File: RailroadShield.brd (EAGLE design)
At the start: 99.6 x 78.7 mm, 68 parts, among them J1 5520250-3, J2 5520250-3, J3 5520250-3, J4 5520426-4, J5 5520426-4, J6 KK-156-5, J7 KK-156-5, J8 MSTB-02, Q1 PMBT2222, U1 LM393N, U2 MCP2515-P, U3 MCP2551-P, U4 MAX3468CPA, U5 MAX3468CPA, U6 MAX3468CPA, U7 LM317LD, U8 6N137, Y1 16Mhz

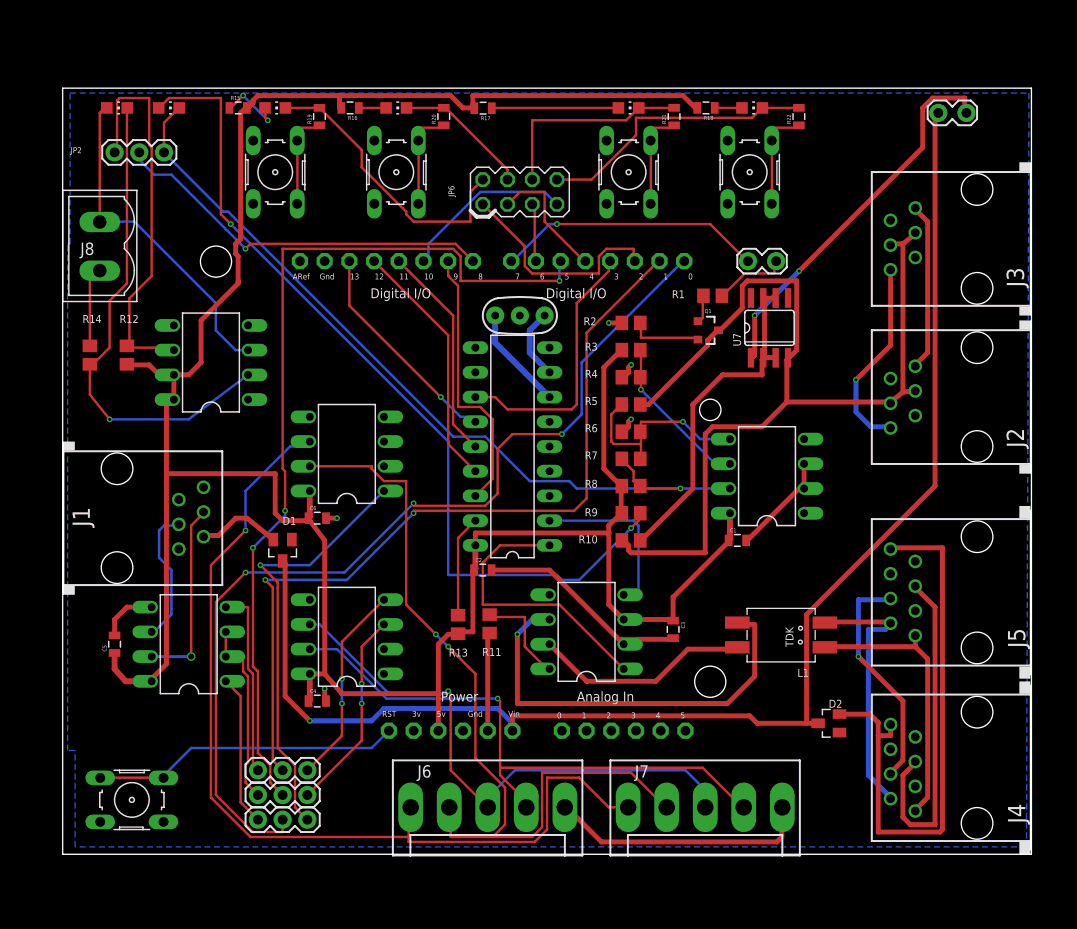
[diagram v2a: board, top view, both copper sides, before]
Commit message: 2.1smd
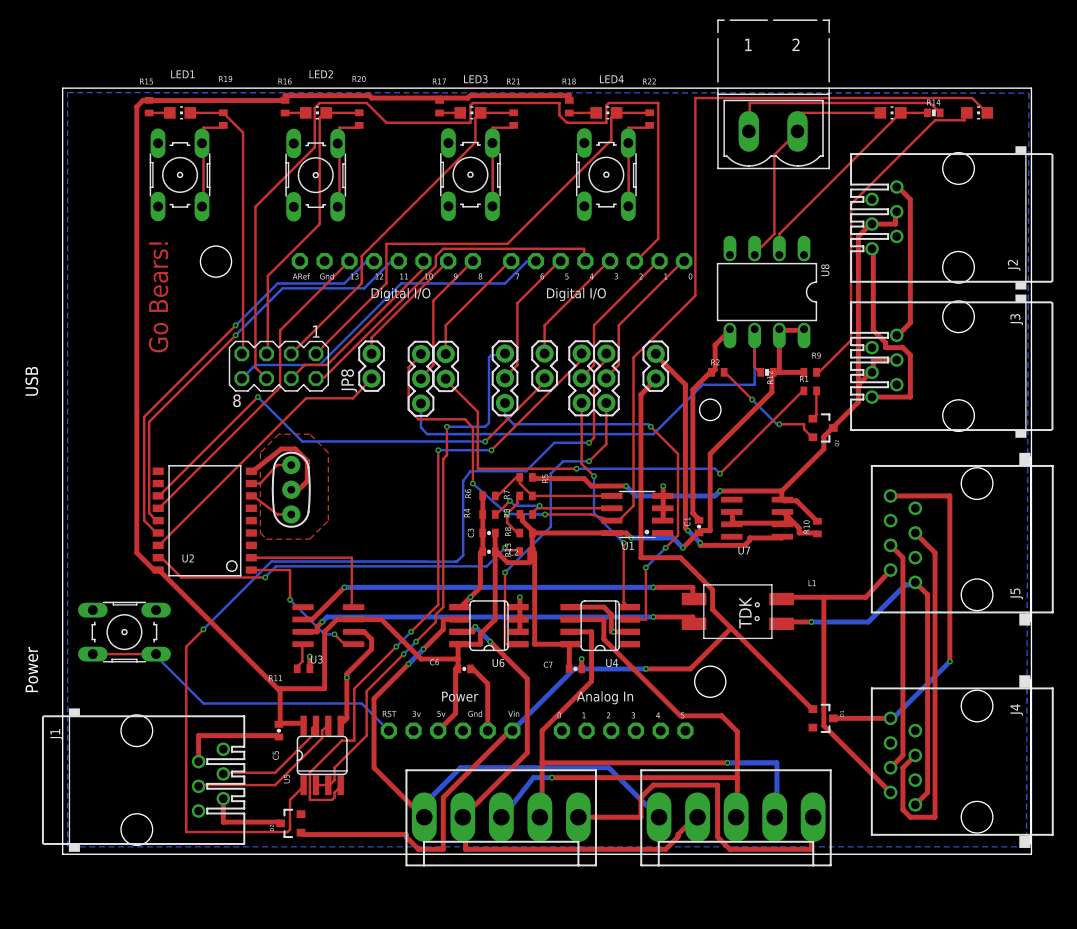
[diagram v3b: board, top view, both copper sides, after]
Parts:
- removed C4: 0.01uf, MCP:0805
- removed J8: MSTB-02, MCP:MSTBV2
- removed Q1: PMBT2222, MCP:SOT23-3
- removed U$1: ARDUINODUEMILANOVE, MCP:ARDUINO-BIGSHIELD
- added C7: .1uF, SparkFun:0402-CAP
- added J9: .200 2-pin, con-phoenix-500:MSTBV2
- added JP8: CAN-CS, SparkFun:1X02
- added JP9: (no value), con-lstb:MA04-2
- added MOD1: ARDUINO DUEMILANOVE, microbuilder:ARDUINO-BIGSHIELD
- added Q2: BC817-16LT1G, SparkFun:SOT23-3
- C1, C2, C3: value 0.01uf -> .1uf; device MCP:0805 -> SparkFun:0402-CAP
- C5, C6: value 0.01uf -> .1uF; device MCP:0805 -> SparkFun:0402-CAP
- D1, D2: value BAV199 -> (none); device diode:SOT23 -> SparkFun:SOT23-3
- J1, J2, J3: value 5520250-3 -> RJ12; device MCP:RJ11-NO_SHIELD -> con-amp:520250-3
- J4, J5: value 5520426-4 -> RJ45; device MCP:RJ45-NO-SHIELD -> con-tycoelectronics:RJ45-NO-SHIELD
- J6: value KK-156-5 -> 5-pin molex; device MCP:KK-156-5 -> con-molex:KK-156-5
- J7: value KK-156-5 -> 5-pin Molex; device MCP:KK-156-5 -> con-molex:KK-156-5
- JP1: value LN-TERM -> LN_TERM; device MCP:1X02_LOCK -> SparkFun:1X02
- JP2: device MCP:1X03 -> SparkFun:1X03
- JP3: value RxD -> CAN-INT; device MCP:1X03 -> SparkFun:1X02
- JP4: value EN -> TXD; device MCP:1X03 -> SparkFun:1X02
- JP5: value TxD -> RXD; device MCP:1X03 -> SparkFun:1X03
- JP6: value MA04-2 -> EN; device MCP:MA04-2 -> SparkFun:1X03
- JP7: value LNTX -> TXD; device MCP:1X02_LOCK -> SparkFun:1X03
- LED3, LED4: value Green -> Red
- R1, R10, R11, R13, R3, R4, R5, R6, R7, R8: device rcl:R0805 -> rcl:R0402
- R12: device rcl:R0805 -> SparkFun:0402-RES
- R14: value 1k -> 1K; device rcl:R0805 -> SparkFun:0402-RES
- R15, R16, R17, R18, R19, R20, R21, R22: value 660R -> 680R; device MCP:0805 -> rcl:R0402
- R2: value 18R -> 15R; device rcl:R0805 -> rcl:R0402
- R9: value 1k -> 1K; device rcl:R0805 -> rcl:R0402
- S1, S2, S3, S4: value B3F-1052 -> 611-PTS645SH70LFS; device MCP:B3F-10XX -> switch-omron:B3F-10XX
- S5: value B3F-1000 -> (none); device MCP:B3F-10XX -> switch-omron:B3F-10XX
- U1: value LM393N -> LM393M; device MCP:DIL08 -> MCP:SO08
- U2: value MCP2515-P -> MCP2515-SO; device MCP:DIL18 -> MCP:SO-18W
- U3: value MCP2551-P -> MCP2551-SN; device MCP:DIL08 -> MCP:SO-08
- U4, U5, U6: value MAX3468CPA -> MAX3468CSA; device MCP:DIL08 -> maxim:SO08
- U7: value LM317LD -> LM317LM; device MCP:SO08 -> linear:SO08
- Y1: device MCP:RESONATOR-PTH -> SparkFun:RESONATOR-PTH
- moved R14 90.2 mm to (89.5, 76.2), turned to 180 degrees
- moved LED6 83.1 mm to (94.0, 76.2)
- moved LED5 79.5 mm to (85.1, 76.2)
- moved R12 65.8 mm to (72.4, 49.5), turned to 0 degrees
- moved D1 58.1 mm to (78.1, 14.0), turned to 270 degrees
- moved U8 57.6 mm to (72.4, 57.8), turned to 180 degrees
- moved D2 56.2 mm to (23.5, 3.17)
- moved JP3 51.5 mm to (49.5, 48.9), turned to 90 degrees
- moved JP5 48.7 mm to (55.9, 46.4), turned to 90 degrees
- moved JP4 47.5 mm to (39.4, 51.4), turned to 270 degrees
- moved JP2 40.7 mm to (36.8, 46.3), turned to 90 degrees
- moved JP1 40.3 mm to (61.0, 51.4), turned to 270 degrees
- moved U2 32.5 mm to (14.6, 34.3)
- moved Y1 29.5 mm to (23.5, 37.5), turned to 90 degrees
- moved J1 27.0 mm to (7.62, 7.62)
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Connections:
- net N$10 renamed +IN
- net N$12 renamed OSC1
- net N$13 renamed OSC2
- net N$2 renamed L2+
- net N$3 renamed L3+
- net N$4 renamed L4+
- net N$5 renamed L1+
- net N$6 renamed SHIELD
- net N$7 renamed -OUT
- net N$8 renamed +OUT
- net N$9 renamed -IN
- removed net N$11: J8.1, R14.1
- new net CAN-CS: JP8.1, U2.16
- new net CAN-INT: JP3.1, U2.12
- new net DCCA: J9.1, R14.1
- net 3V: now also MOD1.3V; no longer U$1.3V
- net A/RESET: now also MOD1.RESET; no longer U$1.RESET
- net CAN-PWR+: now also D1.3; no longer D2.2
- net CMRIRX: now also JP5.1; no longer JP3.1
- net CMRITX: now also JP7.1; no longer JP5.1
- net CMRITXEN: now also JP6.1; no longer JP4.1
- net D0: now also JP5.2, MOD1.D0; no longer JP3.2, U$1.D0
- net D1: now also JP7.2, MOD1.D1; no longer JP5.2, U$1.D1
- net D10: now also JP9.4, MOD1.D10; no longer JP6.7, U$1.D10
- net D11: now also MOD1.D11; no longer U$1.D11
- net D12: now also MOD1.D12; no longer U$1.D12
- net D13: now also MOD1.D13; no longer U$1.D13
- net D2: now also JP9.6, MOD1.D2; no longer JP6.1, U$1.D2
- net D3: now also JP3.2, MOD1.D3; no longer U$1.D3, U2.12
- net D4: now also JP9.2, MOD1.D4; no longer JP6.3, U$1.D4
- net D5: now also JP6.2, MOD1.D5; no longer JP4.2, U$1.D5
- net D6: now also JP9.8, MOD1.D6; no longer JP6.5, U$1.D6
- net D7: now also JP4.1, MOD1.D7; no longer JP7.2, U$1.D7
- net D8: now also MOD1.D8; no longer U$1.D8
- net D9: now also JP8.2, MOD1.D9; no longer U$1.D9, U2.16
- net DCCB: now also J9.2; no longer J8.2
- net GND: now also C7.2, MOD1.GND, MOD1.GND1, MOD1.GND2; no longer C4.2, U$1.GND, U$1.GND1, U$1.GND2
- net IO1: now also JP9.7; no longer JP6.2
- net IO2: now also JP9.5; no longer JP6.4
- net IO3: now also JP9.3; no longer JP6.6
- net IO4: now also JP9.1; no longer JP6.8
- net LN-TX: now also Q2.1; no longer Q1.1
- net LNTX: now also JP4.2; no longer JP7.1
- net LOCONET: now also Q2.3; no longer Q1.3
- net N$1: now also Q2.2; no longer Q1.2
- net NCE-PWR+: now also D2.3; no longer D1.2
- net NCERX: now also JP5.3; no longer JP3.3
- net NCETX: now also JP7.3; no longer JP5.3
- net NCETXEN: now also JP6.3; no longer JP4.3
- net V+: now also D1.1, D2.1, MOD1.VIN; no longer D1.3, D2.3, U$1.VIN
- net VCC: now also C7.1, MOD1.5V; no longer C4.1, U$1.5V
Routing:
- net NCERX: track 15.6 -> 99.5 mm, vias 0 -> 2
- net D0: track 98.3 -> 15.4 mm, vias 3 -> 0
- net D5: track 92.3 -> 14.5 mm, vias 3 -> 0
- net D1: track 84.5 -> 15.4 mm, vias 2 -> 0
- net D2: track 23.1 -> 89.9 mm
- net L6+: track 88.7 -> 35.1 mm, vias 2 -> 0
- net CAN-INT: track 0.00 -> 48.7 mm, vias 0 -> 2
- net NCETX: track 19.5 -> 65.5 mm, vias 0 -> 4
- net +IN: track 97.1 -> 56.3 mm, vias 1 -> 2
- net LNTX: track 7.79 -> 47.8 mm, vias 0 -> 2
- net V+: track 142.0 -> 102.0 mm
- net GND: track 56.9 -> 94.8 mm, vias 5 -> 7
- net NCETXEN: track 19.4 -> 56.3 mm, vias 0 -> 3
- net LNRX: track 85.9 -> 118.1 mm, vias 1 -> 3
- net -IN: track 84.9 -> 55.5 mm
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- added copper zone on layer 1, net GND
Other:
- board text added: "16Mhz"
- board text added: "2010.10"
- board text added: "Activity"
- board text added: "CAN-CS"
- board text added: "D3"
- board text added: "D9"
- board text added: "Designed in the PCR / Coast Division / NMRA"
- board text added: "RXD"
- board text added: "Railroad"
- board text added: "Rev. 2.1smd"
- board text added: "Switches"
- board text added: "Termination"
- board text added: "layout interface"
- board text added: "shield"
- board text removed: ""Go Bears!""
- board text removed: "15mA Loconet Termination"
- board text removed: "2012.03"
- board text removed: "Railroadshield"
- board text removed: "Rev. 2.1"
- board text removed: "So then it's up with the Blue and Gold, Down with the Red..."
- board text removed: "layout interface board"

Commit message: 2.2
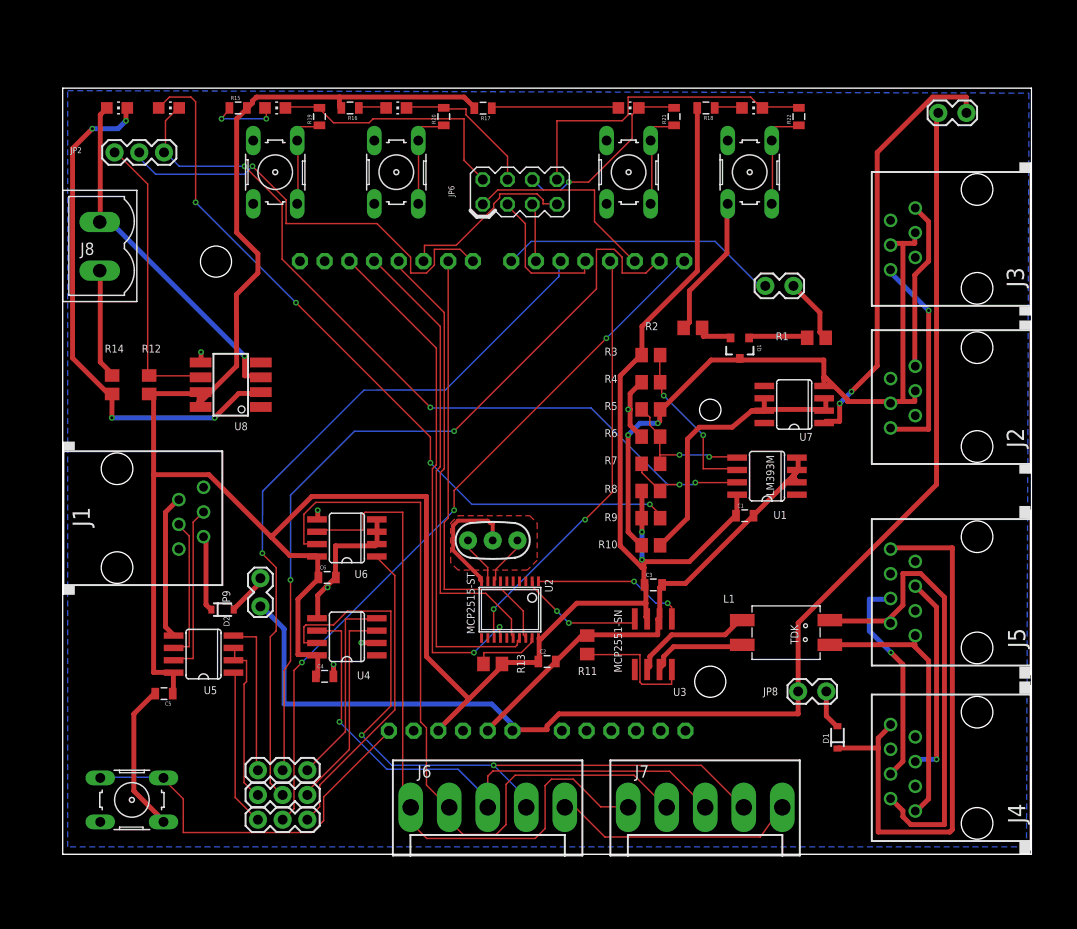
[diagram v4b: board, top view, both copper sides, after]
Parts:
- removed C7: .1uF, SparkFun:0402-CAP
- removed J9: .200 2-pin, con-phoenix-500:MSTBV2
- removed MOD1: ARDUINO DUEMILANOVE, microbuilder:ARDUINO-BIGSHIELD
- removed Q2: BC817-16LT1G, SparkFun:SOT23-3
- added C4: 0.01uf, MCP:0805
- added J8: MSTB-02, MCP:MSTBV2
- added Q1: PMBT2222, MCP:SOT23-3
- added U$1: ARDUINODUEMILANOVE, MCP:ARDUINO-BIGSHIELD
- C1, C2, C3: value .1uf -> 0.01uf; device SparkFun:0402-CAP -> MCP:0805
- C5, C6: value .1uF -> 0.01uf; device SparkFun:0402-CAP -> MCP:0805
- D1, D2: value (none) -> 1N4448WT; device SparkFun:SOT23-3 -> MCP:SOD-323
- J1, J2, J3: value RJ12 -> 5520250-3; device con-amp:520250-3 -> MCP:RJ11-NO_SHIELD
- J4, J5: value RJ45 -> 5520426-4; device con-tycoelectronics:RJ45-NO-SHIELD -> MCP:RJ45-NO-SHIELD
- J6: value 5-pin molex -> KK-156-5; device con-molex:KK-156-5 -> MCP:KK-156-5
- J7: value 5-pin Molex -> KK-156-5; device con-molex:KK-156-5 -> MCP:KK-156-5
- JP1: value LN_TERM -> LN-TERM; device SparkFun:1X02 -> MCP:1X02_LOCK
- JP2: device SparkFun:1X03 -> MCP:1X03
- JP3: value CAN-INT -> RxD; device SparkFun:1X02 -> MCP:1X03
- JP4: value TXD -> EN; device SparkFun:1X02 -> MCP:1X03
- JP5: value RXD -> TxD; device SparkFun:1X03 -> MCP:1X03
- JP6: value EN -> MA04-2; device SparkFun:1X03 -> MCP:MA04-2
- JP7: value TXD -> LNTX; device SparkFun:1X03 -> MCP:1X02_LOCK
- JP8: value CAN-CS -> CANPWR; device SparkFun:1X02 -> MCP:1X02_LOCK
- JP9: value (none) -> NCEPWR; device con-lstb:MA04-2 -> MCP:1X02_LOCK
- LED3, LED4: value Red -> Green
- R1, R10, R11, R13, R3, R4, R5, R6, R7, R8: device rcl:R0402 -> rcl:R0805
- R12: device SparkFun:0402-RES -> rcl:R0805
- R14: value 1K -> 1k; device SparkFun:0402-RES -> rcl:R0805
- R15, R16, R17, R18, R19, R20, R21, R22: value 680R -> 660R; device rcl:R0402 -> MCP:0805
- R2: value 15R -> 18R; device rcl:R0402 -> rcl:R0805
- R9: value 1K -> 1k; device rcl:R0402 -> rcl:R0805
- S1, S2, S3, S4: value 611-PTS645SH70LFS -> B3F-1052; device switch-omron:B3F-10XX -> MCP:B3F-10XX
- S5: value (none) -> B3F-1000; device switch-omron:B3F-10XX -> MCP:B3F-10XX
- U2: value MCP2515-SO -> MCP2515-ST; device MCP:SO-18W -> MCP:TSSOP20
- U4, U5, U6: device maxim:SO08 -> MCP:SO08
- U7: value LM317LM -> LM317LCDR; device linear:SO08 -> MCP:SO08
- U8: value 6N137 -> 6N137SD; device optocoupler:DIL08 -> MCP:SM8
- Y1: device SparkFun:RESONATOR-PTH -> MCP:RESONATOR-PTH
- moved R14 89.0 mm to (5.08, 48.3), turned to 270 degrees
- moved LED6 83.1 mm to (10.9, 76.7)
- moved LED5 79.5 mm to (5.59, 76.7)
- moved R12 63.5 mm to (8.89, 48.3), turned to 270 degrees
- moved JP8 56.6 mm to (78.3, 16.7), turned to 180 degrees
- moved U8 55.9 mm to (17.3, 48.3), turned to 90 degrees
- moved JP3 51.5 mm to (25.1, 3.56), turned to 180 degrees
- moved JP5 48.7 mm to (25.1, 8.64), turned to 180 degrees
- moved JP4 47.5 mm to (25.1, 6.10), turned to 180 degrees
- moved JP2 40.7 mm to (5.33, 72.1), turned to 0 degrees
- moved JP1 40.3 mm to (92.7, 76.2), turned to 180 degrees
- moved U3 33.5 mm to (60.7, 21.6), turned to 180 degrees
- moved U2 32.7 mm to (46.0, 25.1), turned to 180 degrees
- moved R11 29.3 mm to (53.9, 21.5), turned to 90 degrees
- moved J1 27.0 mm to (5.59, 34.5)
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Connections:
- net +IN renamed N$10
- net +OUT renamed N$8
- net -IN renamed N$9
- net -OUT renamed N$7
- net L1+ renamed N$5
- net L2+ renamed N$2
- net L3+ renamed N$3
- net L4+ renamed N$4
- net SHIELD renamed N$6
- removed net CAN-CS: JP8.1, U2.16
- removed net CAN-INT: JP3.1, U2.12
- removed net DCCA: J9.1, R14.1
- removed net OSC1: U2.8, Y1.3
- removed net OSC2: U2.7, Y1.1
- new net N$11: J8.1, R14.1
- new net N$12: U2.9, Y1.3
- new net N$13: U2.8, Y1.1
- new net N$14: D2.2, JP9.1
- new net N$15: D1.2, JP8.1
- net /RESET: now also U2.19; no longer U2.17
- net 3V: now also U$1.3V; no longer MOD1.3V
- net A/RESET: now also U$1.RESET; no longer MOD1.RESET
- net CAN-PWR+: now also D1.1; no longer D1.3
- net CMRIRX: now also JP3.1; no longer JP5.1
- net CMRITX: now also JP5.1; no longer JP7.1
- net CMRITXEN: now also JP4.1; no longer JP6.1
- net D0: now also JP3.2, U$1.D0; no longer JP5.2, MOD1.D0
- net D1: now also JP5.2, U$1.D1; no longer JP7.2, MOD1.D1
- net D10: now also JP6.7, U$1.D10; no longer JP9.4, MOD1.D10
- net D11: now also U$1.D11, U2.16; no longer MOD1.D11, U2.14
- net D12: now also U$1.D12, U2.17; no longer MOD1.D12, U2.15
- net D13: now also U$1.D13, U2.14; no longer MOD1.D13, U2.13
- net D2: now also JP6.1, U$1.D2; no longer JP9.6, MOD1.D2
- net D3: now also U$1.D3, U2.13; no longer JP3.2, MOD1.D3
- net D4: now also JP6.3, U$1.D4; no longer JP9.2, MOD1.D4
- net D5: now also JP4.2, U$1.D5; no longer JP6.2, MOD1.D5
- net D6: now also JP6.5, U$1.D6; no longer JP9.8, MOD1.D6
- net D7: now also JP7.2, U$1.D7; no longer JP4.1, MOD1.D7
- net D8: now also U$1.D8; no longer MOD1.D8
- net D9: now also U$1.D9, U2.18; no longer JP8.2, MOD1.D9
- net DCCB: now also J8.2; no longer J9.2
- net GND: now also C4.2, U$1.GND, U$1.GND1, U$1.GND2, U2.10; no longer C7.2, MOD1.GND, MOD1.GND1, MOD1.GND2, U2.9
- net IO1: now also JP6.2; no longer JP9.7
- net IO2: now also JP6.4; no longer JP9.5
- net IO3: now also JP6.6; no longer JP9.3
- net IO4: now also JP6.8; no longer JP9.1
- net LN-TX: now also Q1.1; no longer Q2.1
- net LNTX: now also JP7.1; no longer JP4.2
- net LOCONET: now also Q1.3; no longer Q2.3
- net N$1: now also Q1.2; no longer Q2.2
- net NCE-PWR+: now also D2.1; no longer D2.3
- net NCERX: now also JP3.3; no longer JP5.3
- net NCETX: now also JP5.3; no longer JP7.3
- net NCETXEN: now also JP4.3; no longer JP6.3
- net V+: now also JP8.2, JP9.2, U$1.VIN; no longer D1.1, D2.1, MOD1.VIN
- net VCC: now also C4.1, U$1.5V, U2.20; no longer C7.1, MOD1.5V, U2.18
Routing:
- net NCERX: track 99.5 -> 16.2 mm, vias 2 -> 0
- net D2: track 89.9 -> 21.2 mm
- net D1: track 15.4 -> 81.8 mm, vias 0 -> 2
- net D5: track 14.5 -> 73.9 mm, vias 0 -> 1
- net D0: track 15.4 -> 74.6 mm, vias 0 -> 3
- net NCETX: track 65.5 -> 16.2 mm, vias 4 -> 0
- net CAN-INT: track 48.7 -> 0.00 mm, vias 2 -> 0
- net L6+: track 35.1 -> 77.8 mm, vias 0 -> 4
- net LNTX: track 47.8 -> 6.71 mm, vias 2 -> 0
- net NCETXEN: track 56.3 -> 17.3 mm, vias 3 -> 0
- net VCC: track 244.3 -> 283.1 mm
- net GND: track 94.8 -> 133.1 mm, vias 7 -> 6
- net D9: track 12.8 -> 45.8 mm
- net /RESET: track 39.6 -> 7.00 mm, vias 2 -> 0
- net V+: track 102.0 -> 134.2 mm, vias 1 -> 0
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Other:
- board text added: ""Go Bears!""
- board text added: "Loconet Termination Power"
- board text added: "Railroadshield"
- board text added: "Rev. 2.2"
- board text added: "So then it's up with the Blue and Gold, Down with the Red..."
- board text added: "layout interface board"
- board text removed: "16Mhz"
- board text removed: "Activity"
- board text removed: "CAN-CS"
- board text removed: "D3"
- board text removed: "D9"
- board text removed: "Designed in the PCR / Coast Division / NMRA"
- board text removed: "RXD"
- board text removed: "Railroad"
- board text removed: "Rev. 2.1smd"
- board text removed: "Switches"
- board text removed: "Termination"
- board text removed: "layout interface"
- board text removed: "shield"
